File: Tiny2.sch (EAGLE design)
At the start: 12 parts

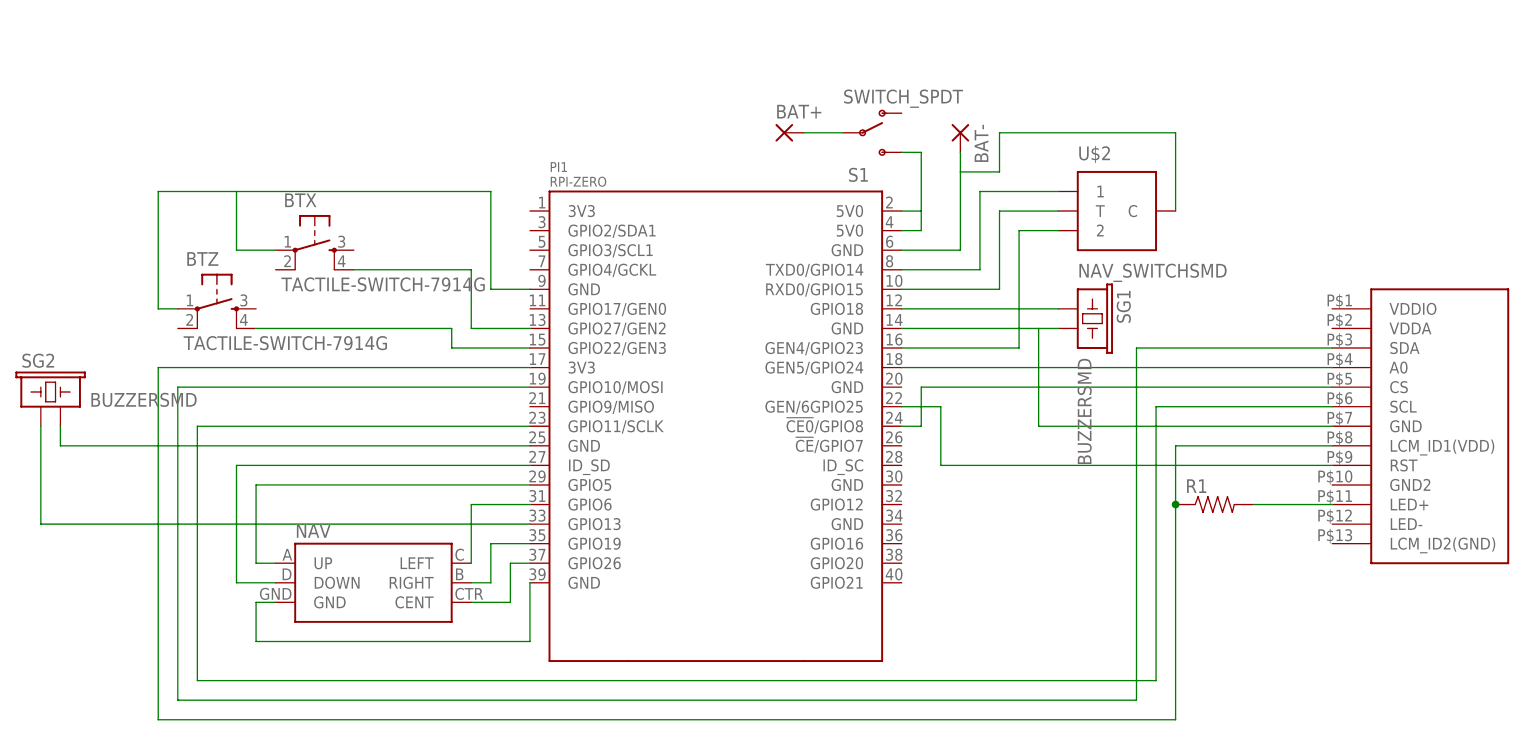
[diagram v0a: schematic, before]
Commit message: Add files via upload
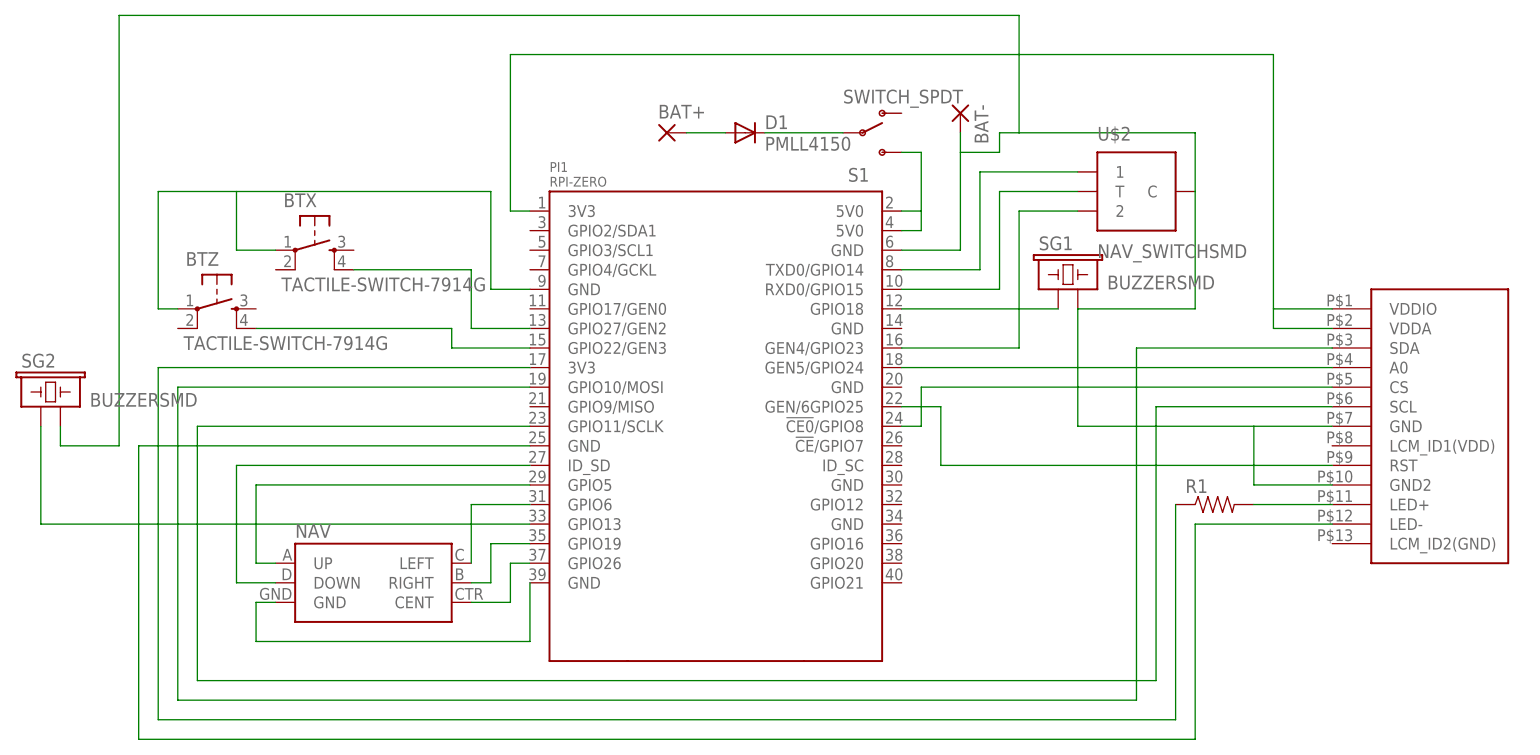
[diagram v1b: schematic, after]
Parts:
- added D1: PMLL4150, diode:PMLL4150
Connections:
- removed net GND@4: PI1.GND@4, SG1.2, U$1.GND
- removed net N$19: PI1.3V3@2, R1.1, U$1.LCM_ID1(VDD)
- removed net N$24: BAT+.P, S1.P
- new net 3V3@1: PI1.3V3@1, U$1.VDDA, U$1.VDDIO
- new net 3V3@2: PI1.3V3@2, R1.1
- new net N$20: BAT+.P, D1.A
- new net N$21: D1.C, S1.P
- net GND@2: now also U$1.LED-; no longer SG2.2
- net GND@8: now also SG1.2, SG2.2, U$1.GND, U$1.GND2
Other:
- moved on the sheet: BAT+, BAT-, SG1, U$2
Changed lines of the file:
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@@
 <part name="SG2" library="SparkFun-Electromechanical" deviceset="BUZZER" device="SMD"/>
 <part name="U$2" library="SparkFun-Electromechanical" deviceset="NAV_SWITCH" device="SMD"/>
+<part name="D1" library="diode" deviceset="PMLL4150" device=""/>
 </parts>
 <sheets>
@@
 <instance part="PI1" gate="G$1" x="0" y="50.8"/>
 <instance part="S1" gate="G$1" x="20.32" y="91.44"/>
-<instance part="BAT+" gate="1" x="10.16" y="91.44"/>
-<instance part="BAT-" gate="1" x="33.02" y="91.44" rot="R270"/>
+<instance part="BAT+" gate="1" x="-5.08" y="91.44"/>
+<instance part="BAT-" gate="1" x="33.02" y="93.98" rot="R270"/>
 <instance part="U$1" gate="G$1" x="91.44" y="53.34" rot="R270"/>
 <instance part="R1" gate="G$1" x="66.04" y="43.18"/>
 <instance part="BTX" gate="G$1" x="-50.8" y="76.2"/>
 <instance part="BTZ" gate="G$1" x="-63.5" y="68.58"/>
-<instance part="SG1" gate="G$1" x="48.26" y="68.58" rot="R270"/>
+<instance part="SG1" gate="G$1" x="45.72" y="71.12"/>
 <instance part="SG2" gate="G$1" x="-86.36" y="55.88"/>
-<instance part="U$2" gate="G$1" x="53.34" y="81.28"/>
+<instance part="U$2" gate="G$1" x="55.88" y="83.82"/>
+<instance part="D1" gate="G$1" x="5.08" y="91.44"/>
 </instances>
 <busses>
@@
 <wire x1="27.94" y1="58.42" x2="27.94" y2="53.34" width="0.1524" layer="91"/>
 <wire x1="27.94" y1="53.34" x2="25.4" y2="53.34" width="0.1524" layer="91"/>
-</segment>
-</net>
-<net name="N$19" class="0">
-<segment>
-<pinref part="PI1" gate="G$1" pin="3V3@2"/>
-<wire x1="-22.86" y1="60.96" x2="-71.12" y2="60.96" width="0.1524" layer="91"/>
-<wire x1="-71.12" y1="60.96" x2="-71.12" y2="15.24" width="0.1524" layer="91"/>
-<pinref part="U$1" gate="G$1" pin="LCM_ID1(VDD)"/>
-<wire x1="-71.12" y1="15.24" x2="60.96" y2="15.24" width="0.1524" layer="91"/>
-<wire x1="60.96" y1="15.24" x2="60.96" y2="43.18" width="0.1524" layer="91"/>
-<pinref part="R1" gate="G$1" pin="1"/>
-<junction x="60.96" y="43.18"/>
-<wire x1="81.28" y1="50.8" x2="60.96" y2="50.8" width="0.1524" layer="91"/>
-<wire x1="60.96" y1="50.8" x2="60.96" y2="43.18" width="0.1524" layer="91"/>
 </segment>
 </net>
@@
 </segment>
 </net>
-<net name="N$24" class="0">
-<segment>
-<pinref part="S1" gate="G$1" pin="P"/>
-<pinref part="BAT+" gate="1" pin="P"/>
-<wire x1="17.78" y1="91.44" x2="12.7" y2="91.44" width="0.1524" layer="91"/>
-</segment>
-</net>
 <net name="GND@8" class="0">
 <segment>
 <pinref part="PI1" gate="G$1" pin="GND@8"/>
 <pinref part="BAT-" gate="1" pin="P"/>
-<wire x1="33.02" y1="88.9" x2="33.02" y2="86.36" width="0.1524" layer="91"/>
-<wire x1="33.02" y1="86.36" x2="33.02" y2="76.2" width="0.1524" layer="91"/>
+<wire x1="33.02" y1="91.44" x2="33.02" y2="88.9" width="0.1524" layer="91"/>
+<wire x1="33.02" y1="88.9" x2="33.02" y2="76.2" width="0.1524" layer="91"/>
 <wire x1="33.02" y1="76.2" x2="25.4" y2="76.2" width="0.1524" layer="91"/>
 <pinref part="U$2" gate="G$1" pin="C"/>
-<wire x1="60.96" y1="81.28" x2="60.96" y2="91.44" width="0.1524" layer="91"/>
-<wire x1="60.96" y1="91.44" x2="38.1" y2="91.44" width="0.1524" layer="91"/>
-<wire x1="38.1" y1="91.44" x2="38.1" y2="86.36" width="0.1524" layer="91"/>
-<wire x1="38.1" y1="86.36" x2="33.02" y2="86.36" width="0.1524" layer="91"/>
-</segment>
-</net>
-<net name="GND@4" class="0">
-<segment>
-<pinref part="PI1" gate="G$1" pin="GND@4"/>
+<wire x1="63.5" y1="83.82" x2="63.5" y2="91.44" width="0.1524" layer="91"/>
+<wire x1="63.5" y1="91.44" x2="40.64" y2="91.44" width="0.1524" layer="91"/>
+<wire x1="40.64" y1="91.44" x2="38.1" y2="91.44" width="0.1524" layer="91"/>
+<wire x1="38.1" y1="91.44" x2="38.1" y2="88.9" width="0.1524" layer="91"/>
+<wire x1="38.1" y1="88.9" x2="33.02" y2="88.9" width="0.1524" layer="91"/>
+<wire x1="63.5" y1="83.82" x2="63.5" y2="68.58" width="0.1524" layer="91"/>
 <pinref part="U$1" gate="G$1" pin="GND"/>
-<wire x1="25.4" y1="66.04" x2="43.18" y2="66.04" width="0.1524" layer="91"/>
-<wire x1="43.18" y1="66.04" x2="45.72" y2="66.04" width="0.1524" layer="91"/>
-<wire x1="43.18" y1="53.34" x2="81.28" y2="53.34" width="0.1524" layer="91"/>
+<wire x1="48.26" y1="53.34" x2="71.12" y2="53.34" width="0.1524" layer="91"/>
 <pinref part="SG1" gate="G$1" pin="2"/>
-<wire x1="43.18" y1="53.34" x2="43.18" y2="66.04" width="0.1524" layer="91"/>
+<wire x1="71.12" y1="53.34" x2="81.28" y2="53.34" width="0.1524" layer="91"/>
+<wire x1="48.26" y1="53.34" x2="48.26" y2="68.58" width="0.1524" layer="91"/>
+<pinref part="U$1" gate="G$1" pin="GND2"/>
+<wire x1="81.28" y1="45.72" x2="71.12" y2="45.72" width="0.1524" layer="91"/>
+<wire x1="71.12" y1="45.72" x2="71.12" y2="53.34" width="0.1524" layer="91"/>
+<wire x1="63.5" y1="68.58" x2="48.26" y2="68.58" width="0.1524" layer="91"/>
+<wire x1="40.64" y1="91.44" x2="40.64" y2="106.68" width="0.1524" layer="91"/>
+<wire x1="-76.2" y1="50.8" x2="-83.82" y2="50.8" width="0.1524" layer="91"/>
+<wire x1="-83.82" y1="50.8" x2="-83.82" y2="53.34" width="0.1524" layer="91"/>
+<pinref part="SG2" gate="G$1" pin="2"/>
+<wire x1="40.64" y1="106.68" x2="-76.2" y2="106.68" width="0.1524" layer="91"/>
+<wire x1="-76.2" y1="106.68" x2="-76.2" y2="50.8" width="0.1524" layer="91"/>
 </segment>
 </net>
@@
 </segment>
 </net>
-<net name="GND@2" class="0">
-<segment>
-<pinref part="PI1" gate="G$1" pin="GND@2"/>
-<wire x1="-22.86" y1="50.8" x2="-83.82" y2="50.8" width="0.1524" layer="91"/>
-<wire x1="-83.82" y1="50.8" x2="-83.82" y2="53.34" width="0.1524" layer="91"/>
-<pinref part="SG2" gate="G$1" pin="2"/>
-</segment>
-</net>
 <net name="N$16" class="0">
 <segment>
 <pinref part="PI1" gate="G$1" pin="TXD0/GPIO14"/>
 <wire x1="25.4" y1="73.66" x2="35.56" y2="73.66" width="0.1524" layer="91"/>
-<wire x1="35.56" y1="73.66" x2="35.56" y2="83.82" width="0.1524" layer="91"/>
+<wire x1="35.56" y1="73.66" x2="35.56" y2="86.36" width="0.1524" layer="91"/>
 <pinref part="U$2" gate="G$1" pin="1"/>
-<wire x1="35.56" y1="83.82" x2="45.72" y2="83.82" width="0.1524" layer="91"/>
+<wire x1="35.56" y1="86.36" x2="48.26" y2="86.36" width="0.1524" layer="91"/>
 </segment>
 </net>
@@
 <pinref part="PI1" gate="G$1" pin="RXD0/GPIO15"/>
 <wire x1="25.4" y1="71.12" x2="38.1" y2="71.12" width="0.1524" layer="91"/>
-<wire x1="38.1" y1="71.12" x2="38.1" y2="81.28" width="0.1524" layer="91"/>
+<wire x1="38.1" y1="71.12" x2="38.1" y2="83.82" width="0.1524" layer="91"/>
 <pinref part="U$2" gate="G$1" pin="T"/>
-<wire x1="38.1" y1="81.28" x2="45.72" y2="81.28" width="0.1524" layer="91"/>
+<wire x1="38.1" y1="83.82" x2="48.26" y2="83.82" width="0.1524" layer="91"/>
 </segment>
 </net>
@@
 <pinref part="PI1" gate="G$1" pin="GEN4/GPIO23"/>
 <wire x1="25.4" y1="63.5" x2="40.64" y2="63.5" width="0.1524" layer="91"/>
-<wire x1="40.64" y1="63.5" x2="40.64" y2="78.74" width="0.1524" layer="91"/>
+<wire x1="40.64" y1="63.5" x2="40.64" y2="81.28" width="0.1524" layer="91"/>
 <pinref part="U$2" gate="G$1" pin="2"/>
-<wire x1="40.64" y1="78.74" x2="45.72" y2="78.74" width="0.1524" layer="91"/>
-</segment>
-</net>
+<wire x1="40.64" y1="81.28" x2="48.26" y2="81.28" width="0.1524" layer="91"/>
+</segment>
+</net>
+<net name="N$20" class="0">
+<segment>
+<pinref part="BAT+" gate="1" pin="P"/>
+<pinref part="D1" gate="G$1" pin="A"/>
+<wire x1="-2.54" y1="91.44" x2="2.54" y2="91.44" width="0.1524" layer="91"/>
+</segment>
+</net>
+<net name="N$21" class="0">
+<segment>
+<pinref part="D1" gate="G$1" pin="C"/>
+<pinref part="S1" gate="G$1" pin="P"/>
+<wire x1="7.62" y1="91.44" x2="17.78" y2="91.44" width="0.1524" layer="91"/>
+</segment>
+</net>
+<net name="3V3@1" class="0">
+<segment>
+<pinref part="PI1" gate="G$1" pin="3V3@1"/>
+<wire x1="-22.86" y1="81.28" x2="-25.4" y2="81.28" width="0.1524" layer="91"/>
+<wire x1="-25.4" y1="81.28" x2="-25.4" y2="101.6" width="0.1524" layer="91"/>
+<wire x1="-25.4" y1="101.6" x2="73.66" y2="101.6" width="0.1524" layer="91"/>
+<wire x1="73.66" y1="101.6" x2="73.66" y2="68.58" width="0.1524" layer="91"/>
+<pinref part="U$1" gate="G$1" pin="VDDIO"/>
+<wire x1="73.66" y1="68.58" x2="81.28" y2="68.58" width="0.1524" layer="91"/>
+<pinref part="U$1" gate="G$1" pin="VDDA"/>
+<wire x1="81.28" y1="66.04" x2="73.66" y2="66.04" width="0.1524" layer="91"/>
+<wire x1="73.66" y1="66.04" x2="73.66" y2="68.58" width="0.1524" layer="91"/>
+</segment>
+</net>
+<net name="3V3@2" class="0">
+<segment>
+<pinref part="R1" gate="G$1" pin="1"/>
+<wire x1="60.96" y1="43.18" x2="60.96" y2="15.24" width="0.1524" layer="91"/>
+<wire x1="60.96" y1="15.24" x2="-71.12" y2="15.24" width="0.1524" layer="91"/>
+<wire x1="-71.12" y1="15.24" x2="-71.12" y2="60.96" width="0.1524" layer="91"/>
+<pinref part="PI1" gate="G$1" pin="3V3@2"/>
+<wire x1="-71.12" y1="60.96" x2="-22.86" y2="60.96" width="0.1524" layer="91"/>
+</segment>
+</net>
+<net name="GND@2" class="0">
+<segment>
+<pinref part="PI1" gate="G$1" pin="GND@2"/>
+<wire x1="-22.86" y1="50.8" x2="-73.66" y2="50.8" width="0.1524" layer="91"/>
+<wire x1="-73.66" y1="50.8" x2="-73.66" y2="12.7" width="0.1524" layer="91"/>
+<pinref part="U$1" gate="G$1" pin="LED-"/>
+<wire x1="63.5" y1="40.64" x2="81.28" y2="40.64" width="0.1524" layer="91"/>
+<wire x1="63.5" y1="12.7" x2="63.5" y2="40.64" width="0.1524" layer="91"/>
+<wire x1="-73.66" y1="12.7" x2="63.5" y2="12.7" width="0.1524" layer="91"/>
+</segment>
+</net>
